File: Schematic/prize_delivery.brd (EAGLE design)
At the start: 100.1 x 43.2 mm, 10 parts, among them Q1 IRL540

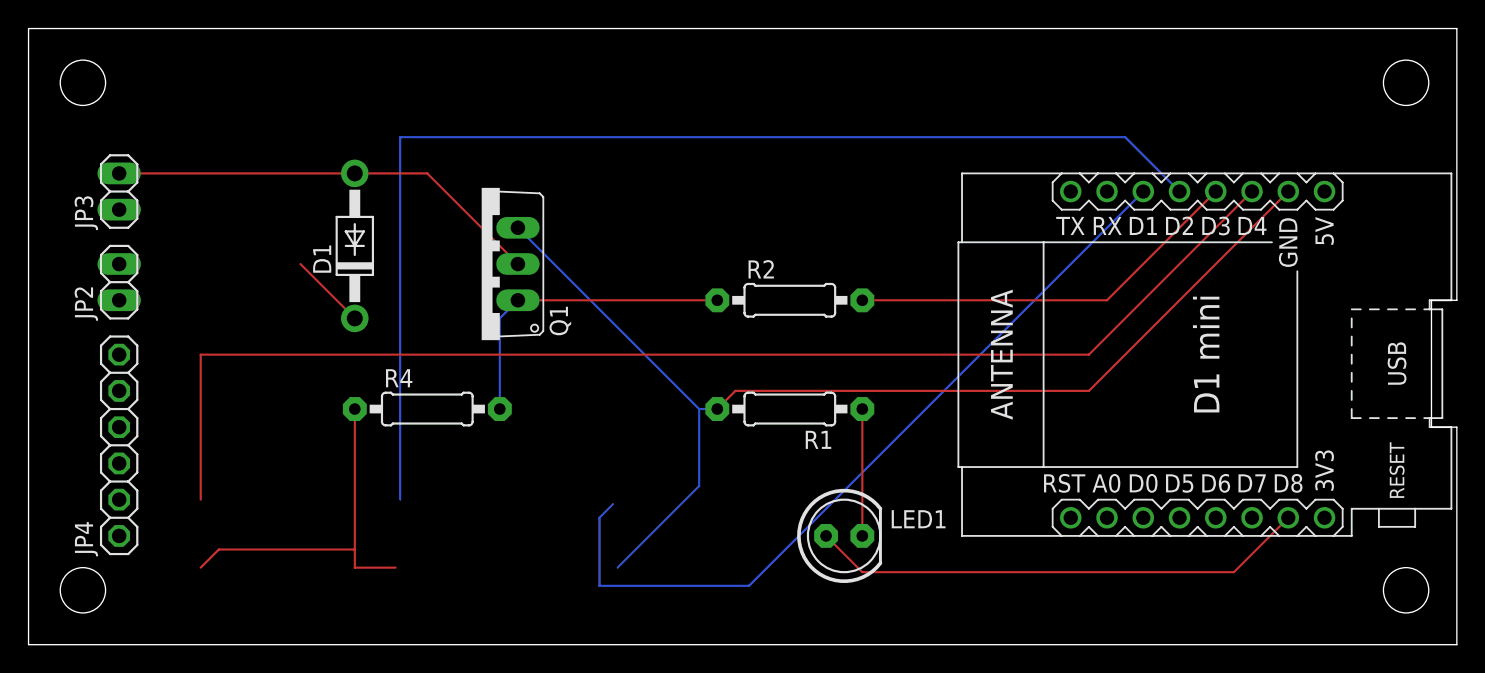
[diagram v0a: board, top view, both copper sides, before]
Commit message: Update PCB
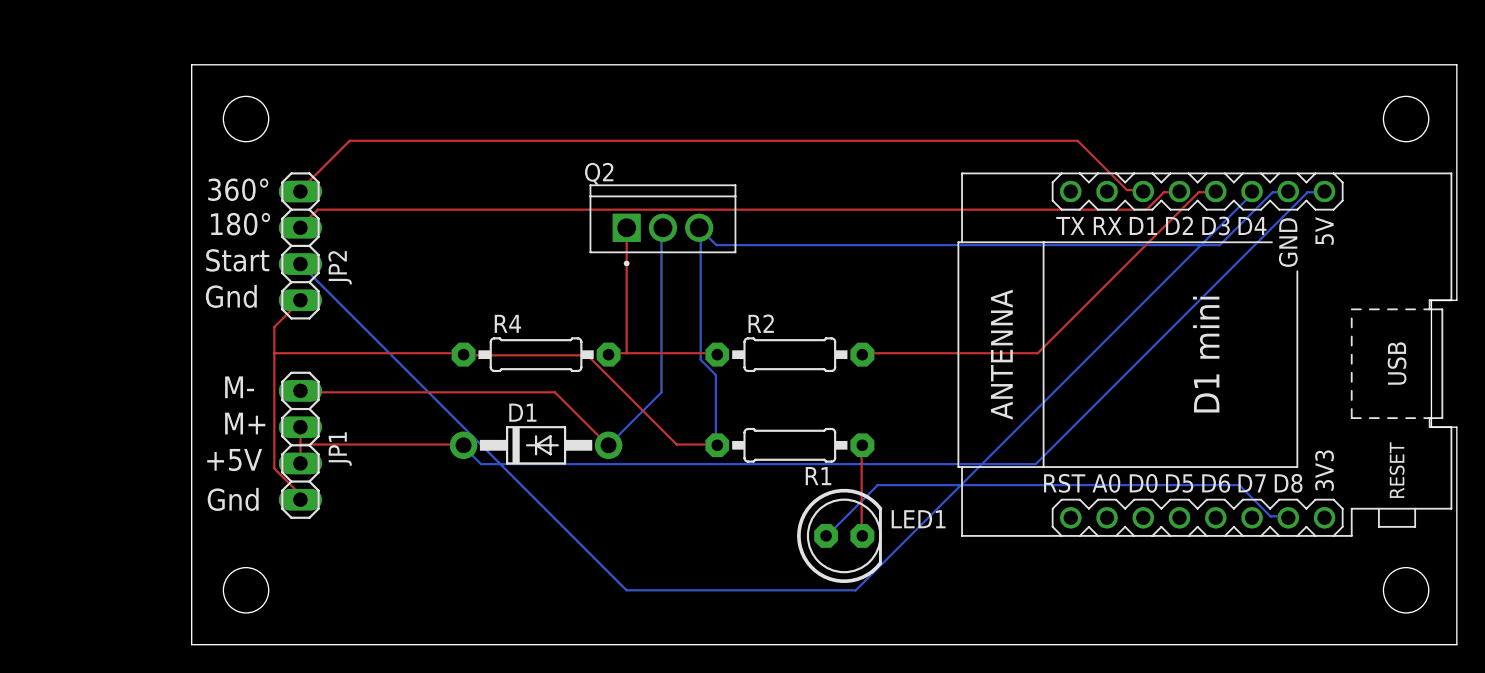
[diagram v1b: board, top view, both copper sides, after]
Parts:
- removed JP3: Motor, pinhead:1X02
- removed JP4: (no value), adafruit:1X06
- removed Q1: IRL540, adafruit:TO220V
- added JP1: (no value), pinhead:1X04
- added Q2: RFP30N06LE, RFP30N06LE:TRANS_RFP30N06LE
- JP2: value 5Vin -> (none); device pinhead:1X02 -> pinhead:1X04
- moved D1 18.9 mm to (35.6, 14.0), turned to 0 degrees
- moved JP2 13.0 mm to (19.1, 27.9)
- moved R4 8.52 mm to (35.6, 20.3)
- moved R2 3.81 mm to (53.3, 20.3)
- moved R1 2.54 mm to (53.3, 14.0)
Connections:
- removed net N$14: Q1.1, R2.1, R4.2
- new net N$8: Q2.1, R2.1, R4.2
- net 0: now also JP1.1, Q2.3; no longer JP4.1, Q1.3
- net N$2: now also JP1.4, Q2.2; no longer JP3.2, Q1.2
- net N$3: now also JP1.2, JP1.3; no longer JP2.2, JP3.1
- net N$4: now also JP2.3; no longer JP4.3
- net N$5: now also JP2.4; no longer JP4.4
- net N$9: now also JP2.2; no longer JP4.2
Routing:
- net N$3: track 5.39 -> 82.9 mm
- net N$14: track 22.1 -> 0.00 mm
- net N$4: track 81.6 -> 62.7 mm
- net N$8: track 0.00 -> 16.5 mm
- net N$2: track 30.6 -> 40.0 mm
- net N$5: track 55.7 -> 62.1 mm
- net 0: track 104.3 -> 108.4 mm
- net N$7: track 8.89 -> 6.41 mm
- net N$1: track 27.9 -> 29.5 mm
- net N$9: track 88.6 -> 87.8 mm
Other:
- board size 100.1 x 43.2 mm -> 88.6 x 40.6 mm
- board text added: "+5V"
- board text added: "180°"
- board text added: "360°"
- board text added: "Gnd"
- board text added: "M+"
- board text added: "M-"
- board text added: "Start"
